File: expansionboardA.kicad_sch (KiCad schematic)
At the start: 63 parts, among them J1 DEBUG, J2 USB_A_Stacked, J3 HDMI_A, J4 FAN, J5 Conn_02x06_Odd_Even, P1 USB_C_Plug, U1 MAX3420EECJ, U2 GPIO_U2, U3 AMS1117-3.3, U4 GPIO_U4, U5 MCP3008T-I/SL, U6 CS4344-CZZR, U7 MAX3421EEHJ+T, Y1 Crystal, Y2 Crystal

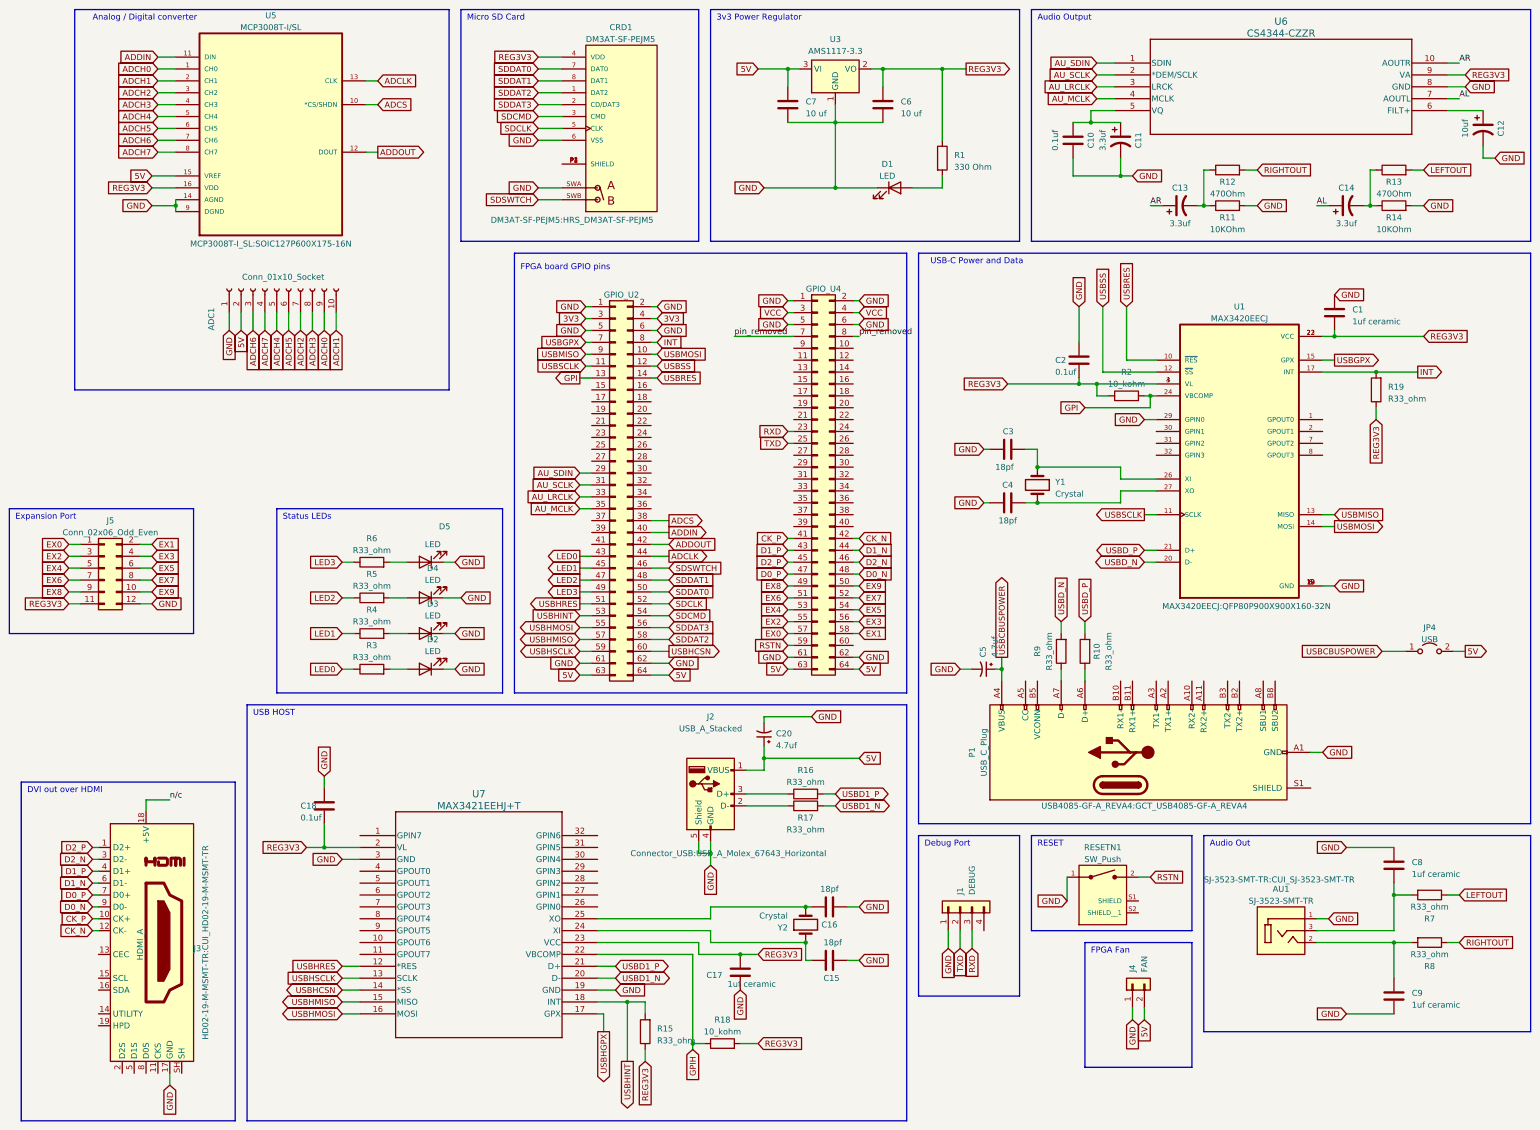
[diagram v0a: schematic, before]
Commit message: Updated board
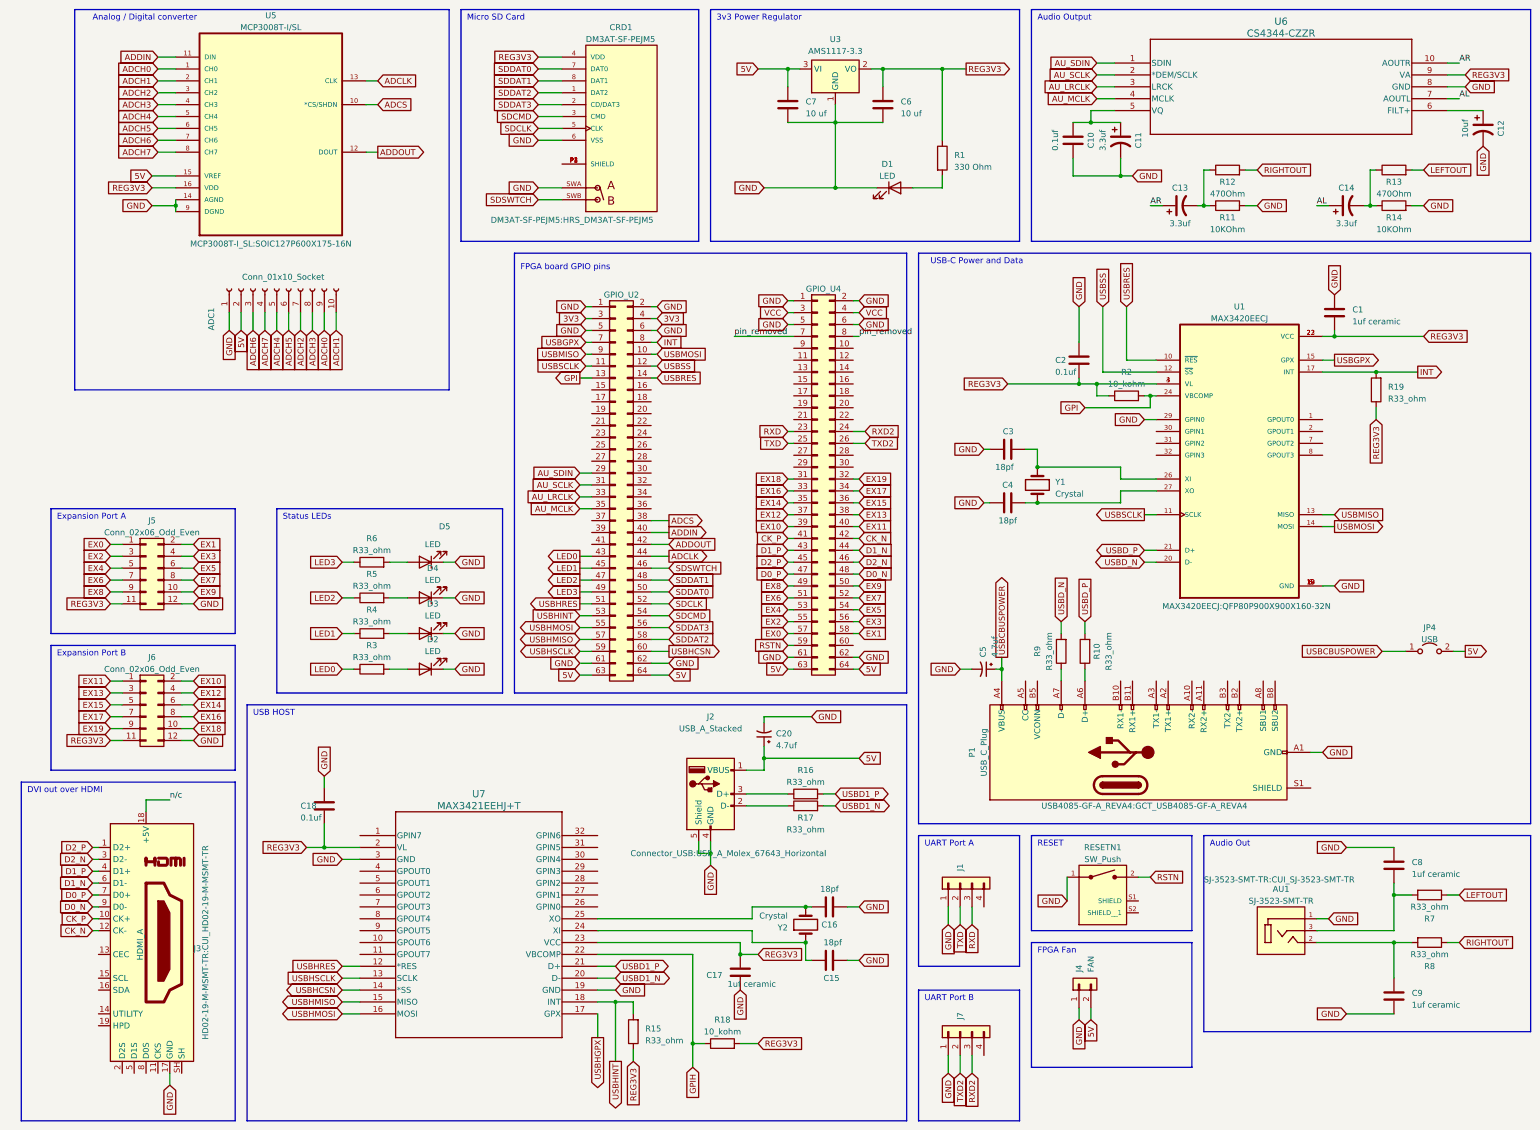
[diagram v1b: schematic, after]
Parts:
- added J6: Conn_02x06_Odd_Even, Connector_PinSocket_2.54mm:PinSocket_2x06_P2.54mm_Vertical, symbol Connector_Generic:Conn_02x06_Odd_Even
- added J7: DEBUG, Connector_PinSocket_2.54mm:PinSocket_1x04_P2.54mm_Vertical, symbol Connector_Generic:Conn_01x04
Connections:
- net GND: now also J6.12 (Pin_12), J7.1 (Pin_1)
- net REG3V3: now also J6.11 (Pin_11)
- net RXD2: now reaches U4.24 (Pin_24)
- net RXD2: now also J7.3 (Pin_3)
- net TXD2: now reaches U4.26 (Pin_26)
- net TXD2: now also J7.2 (Pin_2)
- net EX18: now reaches U4.31 (Pin_31)
- net EX18: now also J6.10 (Pin_10)
- net EX19: now reaches U4.32 (Pin_32)
- net EX19: now also J6.9 (Pin_9)
- net EX16: now reaches U4.33 (Pin_33)
- net EX16: now also J6.8 (Pin_8)
- net EX17: now reaches U4.34 (Pin_34)
- net EX17: now also J6.7 (Pin_7)
- net EX14: now reaches U4.35 (Pin_35)
- net EX14: now also J6.6 (Pin_6)
- net EX15: now reaches U4.36 (Pin_36)
- net EX15: now also J6.5 (Pin_5)
- net EX12: now reaches U4.37 (Pin_37)
- net EX12: now also J6.4 (Pin_4)
- net EX13: now reaches U4.38 (Pin_38)
- net EX13: now also J6.3 (Pin_3)
- net EX10: now reaches U4.39 (Pin_39)
- net EX10: now also J6.2 (Pin_2)
- net EX11: now reaches U4.40 (Pin_40)
- net EX11: now also J6.1 (Pin_1)
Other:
- note added: "Expansion Port A"
- note added: "Expansion Port B"
- note added: "UART Port A"
- note added: "UART Port B"
- note removed: "Debug Port"
- note removed: "Expansion Port"
- moved on the sheet: J1, J4, J5, R15
